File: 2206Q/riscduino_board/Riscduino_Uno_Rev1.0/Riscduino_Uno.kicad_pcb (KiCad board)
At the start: 2 copper layers, 70.6 x 53.7 mm, 93 parts, among them J1 Conn_01x08_Pin, J10 USB_B_Micro, J11 Conn_01x10_Pin, J2 Conn_01x06_Pin, J3 Conn_01x01, J4 Conn_02x04_Odd_Even, J5 ISP, J6 Conn_01x01, J7 Conn_01x01, J8 Conn_01x01, J9 Conn_01x08_Pin, SW1 4Pin Round Button SPST Straig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, U1 MAX1232ESA+T, U2 W25Q32JVSS, U3 W25Q32JVSS, U4 23LC1024-I/P, U5 Riscduino, U6 LM1117MP-3.3, U7 LM1117S-ADJ, U8 CH340C, X1 ASE-10.000MHZ-LC-T

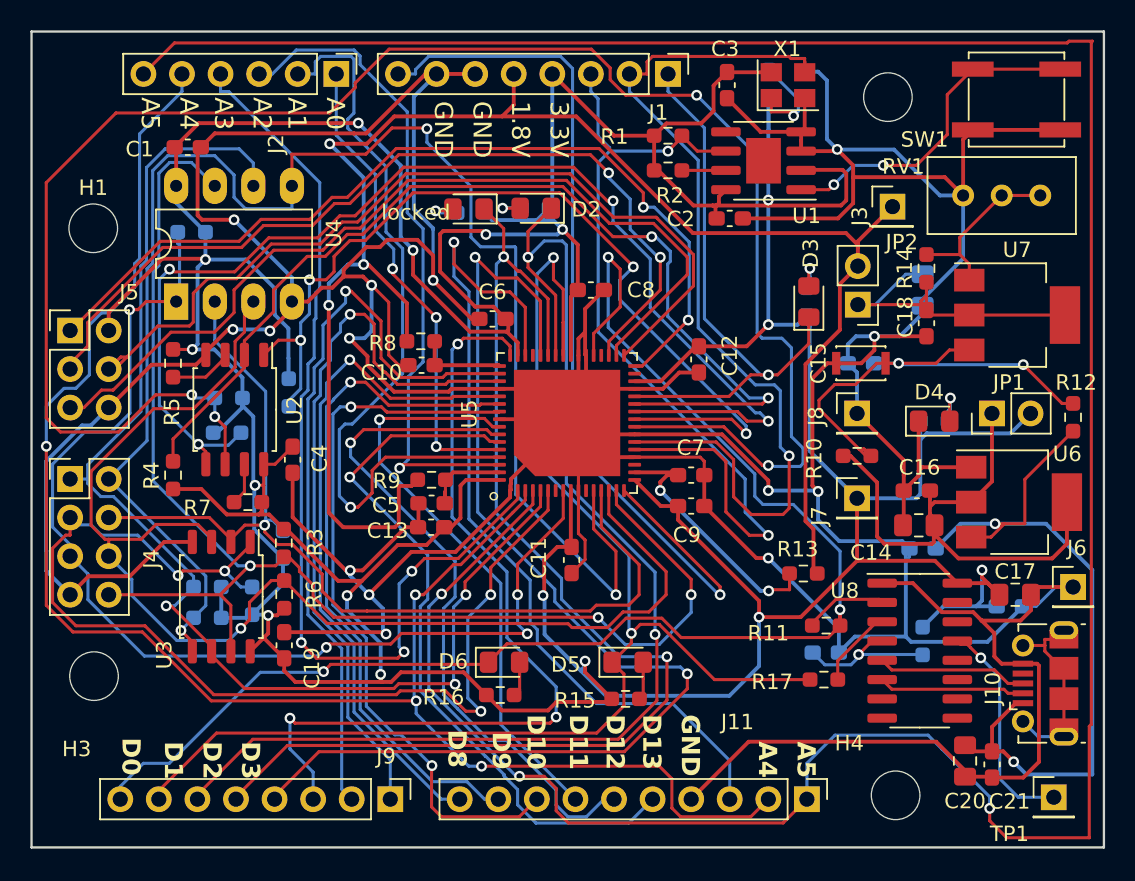
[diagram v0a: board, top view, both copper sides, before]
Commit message: 1.0.9
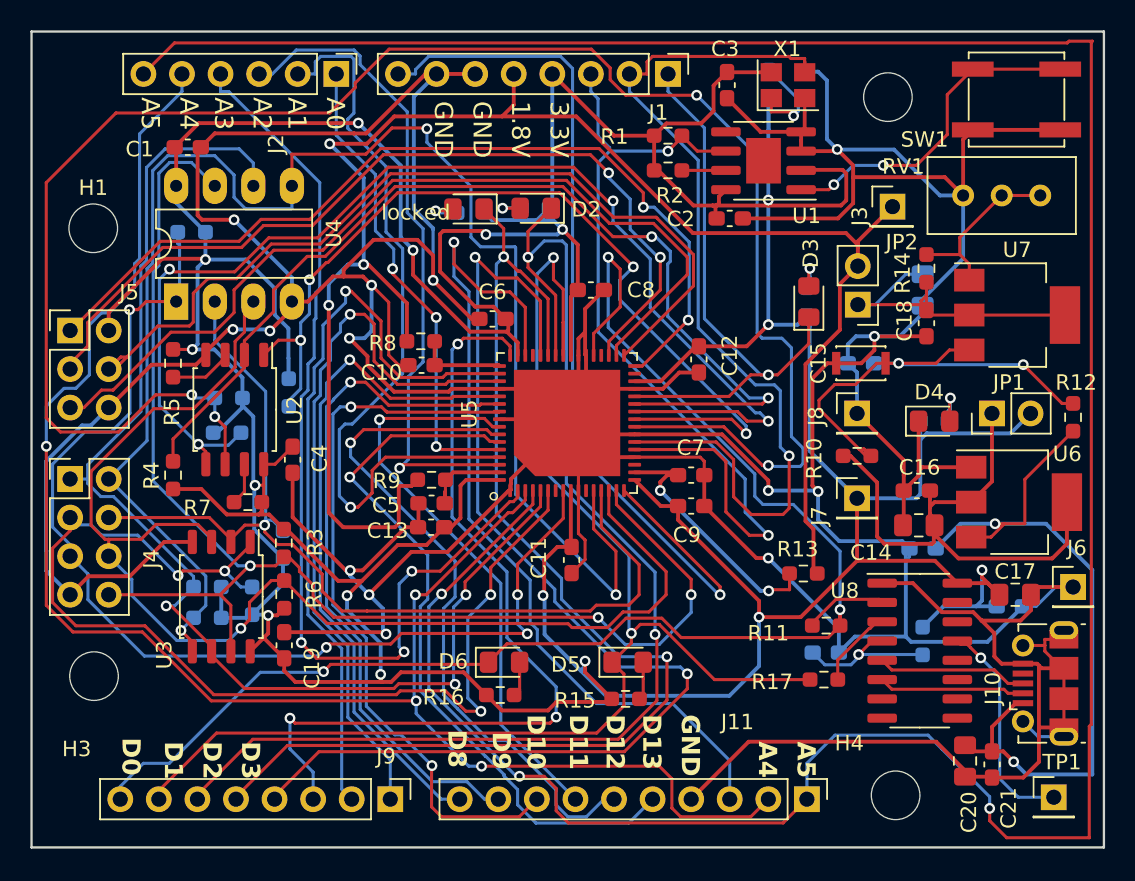
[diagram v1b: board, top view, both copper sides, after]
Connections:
- J10 pad 6: unconnected-(J1-Shield-Pad6) -> GND
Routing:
- net GND: track 449.9 -> 465.0 mm
- net unconnected-(J1-Shield-Pad6): track 11.9 -> 0.00 mm
- net CARAVEL_FLASH_SSN: track 60.2 -> 59.6 mm
